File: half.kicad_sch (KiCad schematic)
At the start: 59 parts, among them SW1 SW_Push, SW13 SW_Push, SW14 SW_Push, SW15 SW_Push, SW16 SW_Push, SW17 SW_Push, SW18 SW_Push, SW25 SW_Push, SW26 SW_Push, SW27 SW_Push, SW28 SW_Push, SW29 SW_Push, SW3 SW_Push, SW30 SW_Push, SW37 SW_Push, SW38 SW_Push, SW39 SW_Push, SW40 SW_Push, SW41 SW_Push, SW42 SW_Push, SW49 SW_Push, SW5 SW_Push, SW50 SW_Push, SW51 SW_Push, SW52 SW_Push, SW53 SW_Push, SW54 RotaryEncoder_Switch, SW7 SW_Push, SW8 SW_Push, SW9 SW_Push

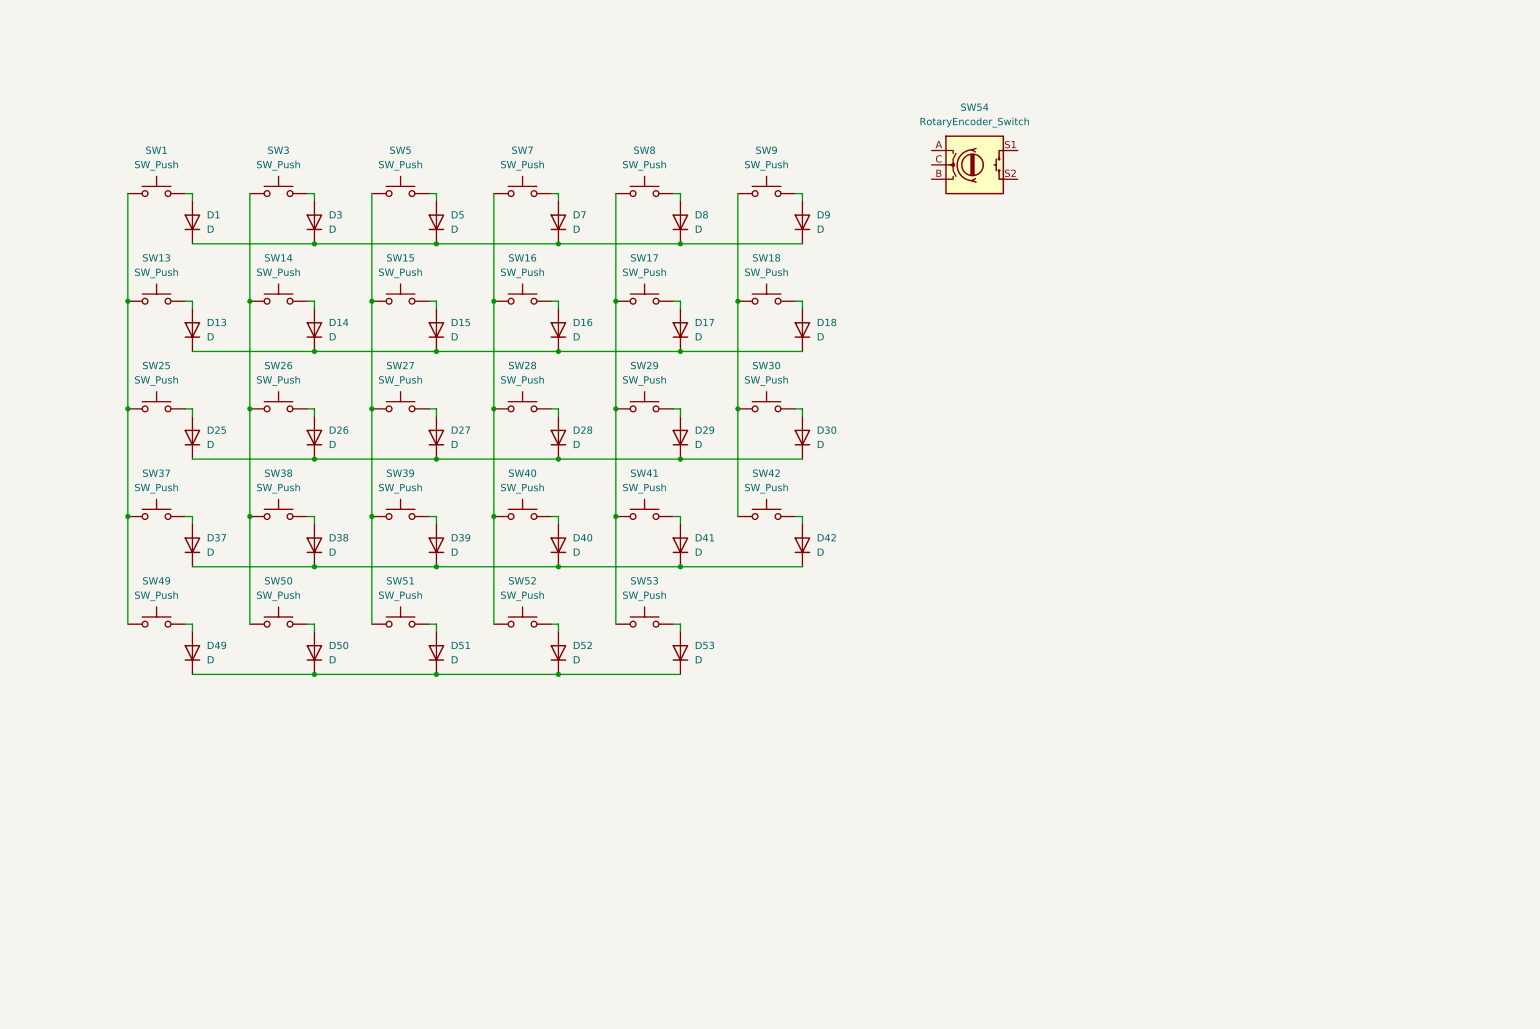
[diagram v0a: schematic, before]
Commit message: Update
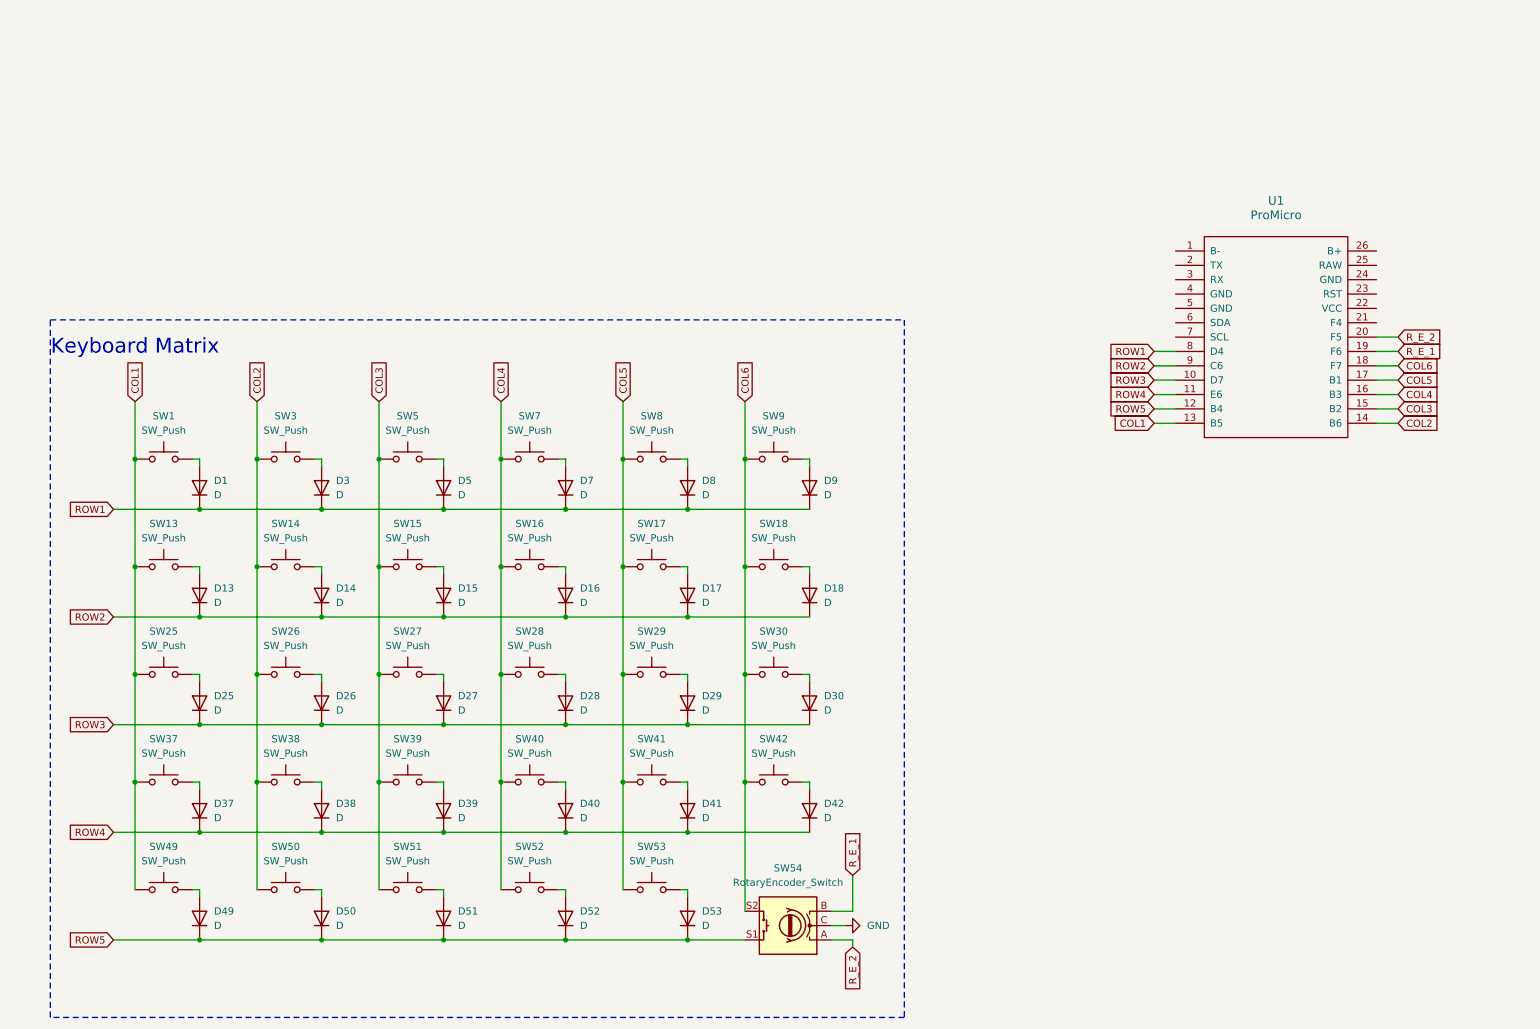
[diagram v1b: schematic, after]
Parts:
- added U1: ProMicro, symbol ProMicro:ProMicro
- D1, D13, D14, D15, D16, D17, D18, D25, D26, D27, D28, D29, D3, D30, D37, D38, D39, D40, D41, D42, D49, D5, D50, D51, D52, D53, D7, D8, D9: footprint (none) -> Diode_SMD:D_SOD-123
- SW1, SW3: footprint (none) -> marbastlib-choc:SW_choc_v1_1u
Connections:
- net ROW4: now reaches D37.1 (K), D38.1 (K), D39.1 (K), D40.1 (K), D41.1 (K), D42.1 (K)
- net ROW4: now also U1.11 (E6)
- net ROW2: now reaches D13.1 (K), D14.1 (K), D15.1 (K), D16.1 (K), D17.1 (K), D18.1 (K)
- net ROW2: now also U1.9 (C6)
- net ROW5: now reaches D49.1 (K), D50.1 (K), D51.1 (K), D52.1 (K), D53.1 (K)
- net ROW5: now also SW54.S1, U1.12 (B4)
- net COL5: now reaches SW17.1, SW29.1, SW41.1, SW53.1, SW8.1
- net COL5: now also U1.17 (B1)
- net ROW1: now reaches D1.1 (K), D3.1 (K), D5.1 (K), D7.1 (K), D8.1 (K), D9.1 (K)
- net ROW1: now also U1.8 (D4)
- net COL3: now reaches SW15.1, SW27.1, SW39.1, SW5.1, SW51.1
- net COL3: now also U1.15 (B2)
- net COL4: now reaches SW16.1, SW28.1, SW40.1, SW52.1, SW7.1
- net COL4: now also U1.16 (B3)
- net COL2: now reaches SW14.1, SW26.1, SW3.1, SW38.1, SW50.1
- net COL2: now also U1.14 (B6)
- net ROW3: now reaches D25.1 (K), D26.1 (K), D27.1 (K), D28.1 (K), D29.1 (K), D30.1 (K)
- net ROW3: now also U1.10 (D7)
- net COL6: now reaches SW18.1, SW30.1, SW42.1, SW9.1
- net COL6: now also SW54.S2, U1.18 (F7)
- net COL1: now reaches SW1.1, SW13.1, SW25.1, SW37.1, SW49.1
- net COL1: now also U1.13 (B5)
- net R_E_2: now reaches SW54.A
- net R_E_2: now also U1.20 (F5)
- net R_E_1: now reaches SW54.B
- net R_E_1: now also U1.19 (F6)
- net GND: now reaches SW54.C
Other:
- note added: "Keyboard Matrix"
- moved on the sheet: D1, D13, D14, D15, D16, D17, D18, D25, D26, D27, D28, D29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

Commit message: Update
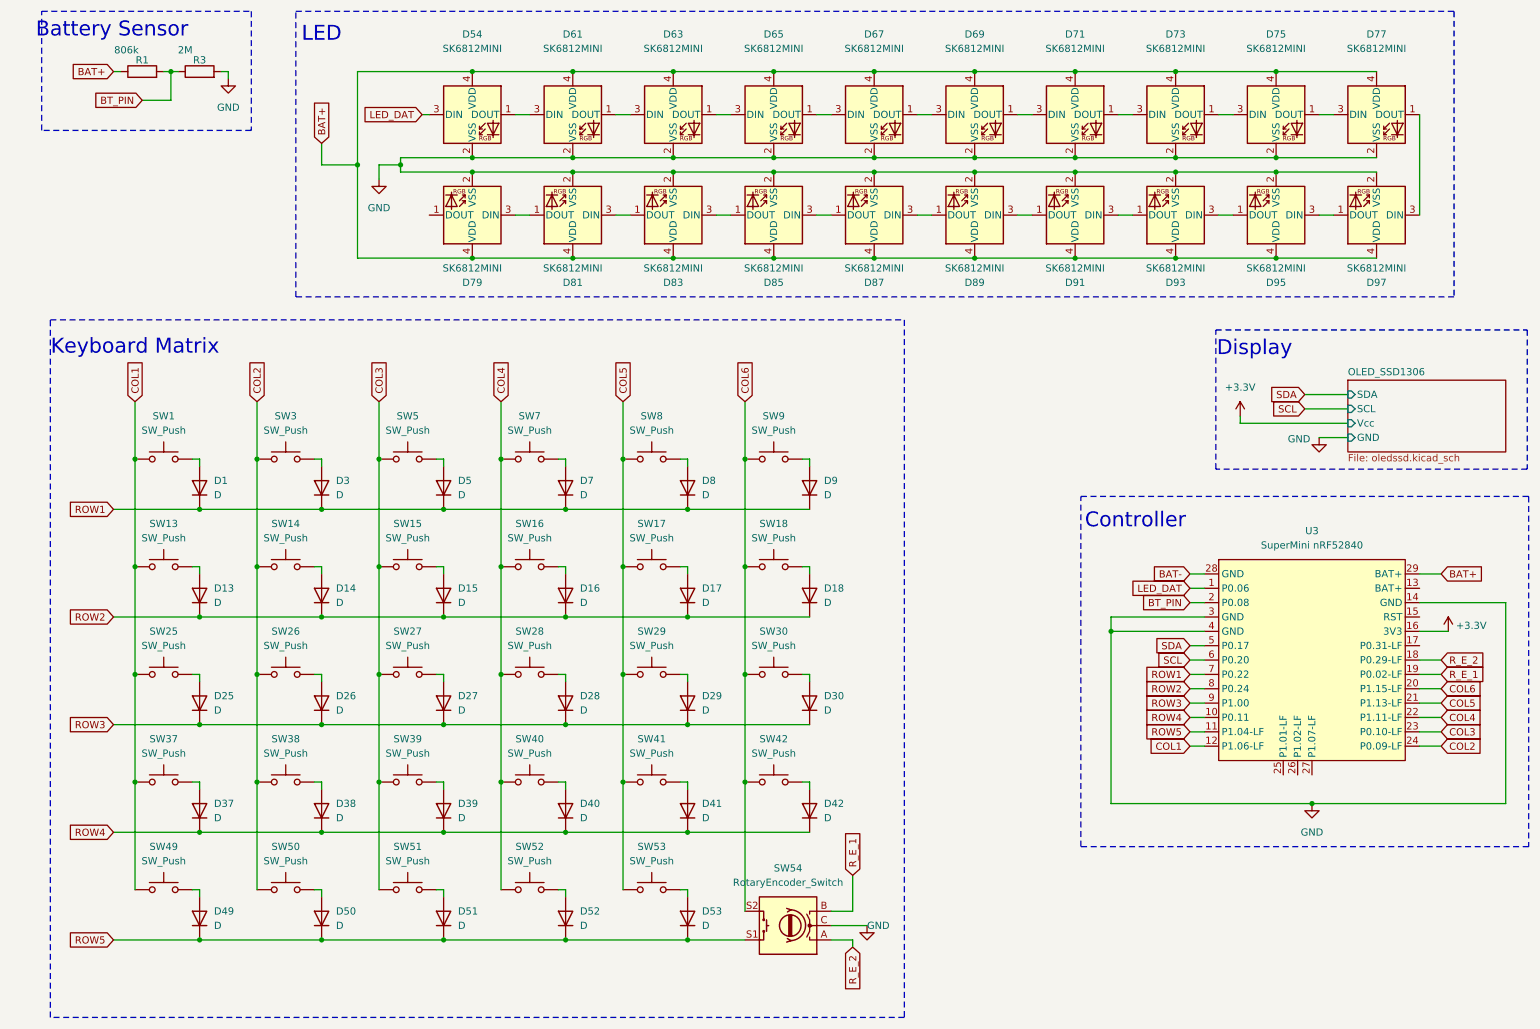
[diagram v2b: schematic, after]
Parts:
- removed U1: ProMicro, symbol ProMicro:ProMicro
- added D54, D61, D63, D65, D67, D69, D71, D73, D75, D77, D79, D81, D83, D85, D87, D89, D91, D93, D95, D97: SK6812MINI, LED_SMD:LED_SK6812MINI_PLCC4_3.5x3.5mm_P1.75mm, symbol LED:SK6812MINI
- added R1: 806k, symbol Device:R
- added R3: 2M, symbol Device:R
- added U3: SuperMini nRF52840, marbastlib-xp-promicroish:SuperMini_nRF52840_AH_USBup, symbol marbastlib-promicroish:SuperMini_nRF52840
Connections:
- net COL1: now also U3.12 (P1.06-LF)
- net COL2: now also U3.24 (P0.09-LF)
- net COL3: now also U3.23 (P0.10-LF)
- net COL4: now also U3.22 (P1.11-LF)
- net COL5: now also U3.21 (P1.13-LF)
- net COL6: now also U3.20 (P1.15-LF)
- net GND: now also D54.2 (VSS), D61.2 (VSS), D63.2 (VSS), D65.2 (VSS), D67.2 (VSS), D69.2 (VSS), D71.2 (VSS), D73.2 (VSS), D75.2 (VSS), D77.2 (VSS), D79.2 (VSS), D81.2 (VSS), D83.2 (VSS), D85.2 (VSS), D87.2 (VSS), D89.2 (VSS), D91.2 (VSS), D93.2 (VSS), D95.2 (VSS), D97.2 (VSS), R3.2, U3.14 (GND), U3.3 (GND), U3.4 (GND)
- net ROW1: now also U3.7 (P0.22)
- net ROW2: now also U3.8 (P0.24)
- net ROW3: now also U3.9 (P1.00)
- net ROW4: now also U3.10 (P0.11)
- net ROW5: now also U3.11 (P1.04-LF)
- net R_E_1: now also U3.19 (P0.02-LF)
- net R_E_2: now also U3.18 (P0.29-LF)
- new net: D87.3 (DIN), D89.1 (DOUT)
- new net: D89.3 (DIN), D91.1 (DOUT)
- new net: D61.1 (DOUT), D63.3 (DIN)
- new net: D54.1 (DOUT), D61.3 (DIN)
- new net: D67.1 (DOUT), D69.3 (DIN)
- new net: D65.1 (DOUT), D67.3 (DIN)
- new net: D81.3 (DIN), D83.1 (DOUT)
- new net: D83.3 (DIN), D85.1 (DOUT)
- new net: D75.1 (DOUT), D77.3 (DIN)
- new net: D73.1 (DOUT), D75.3 (DIN)
- new net: D71.1 (DOUT), D73.3 (DIN)
- new net: D69.1 (DOUT), D71.3 (DIN)
- new net: D79.3 (DIN), D81.1 (DOUT)
- new net: D85.3 (DIN), D87.1 (DOUT)
- new net: D63.1 (DOUT), D65.3 (DIN)
- new net: D91.3 (DIN), D93.1 (DOUT)
- new net: D93.3 (DIN), D95.1 (DOUT)
- new net: D77.1 (DOUT), D97.3 (DIN)
- new net: D95.3 (DIN), D97.1 (DOUT)
- new net +3.3V: U3.16 (3V3)
- new net BAT+: D54.4 (VDD), D61.4 (VDD), D63.4 (VDD), D65.4 (VDD), D67.4 (VDD), D69.4 (VDD), D71.4 (VDD), D73.4 (VDD), D75.4 (VDD), D77.4 (VDD), D79.4 (VDD), D81.4 (VDD), D83.4 (VDD), D85.4 (VDD), D87.4 (VDD), D89.4 (VDD), D91.4 (VDD), D93.4 (VDD), D95.4 (VDD), D97.4 (VDD), R1.1, U3.29 (BAT+)
- new net BAT-: U3.28 (GND)
- new net BT_PIN: R1.2, R3.1, U3.2 (P0.08)
- new net LED_DAT: D54.3 (DIN), U3.1 (P0.06)
- new net SCL: U3.6 (P0.20)
- new net SDA: U3.5 (P0.17)
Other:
- added sheet OLED_SSD1306 (oledssd.kicad_sch)
- note added: "Battery Sensor"
- note added: "Controller"
- note added: "Display"
- note added: "LED"
- title: (none) -> Keyboard Half
